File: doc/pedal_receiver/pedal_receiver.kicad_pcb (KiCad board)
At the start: 2 copper layers, 77 x 17.5 mm, 8 parts

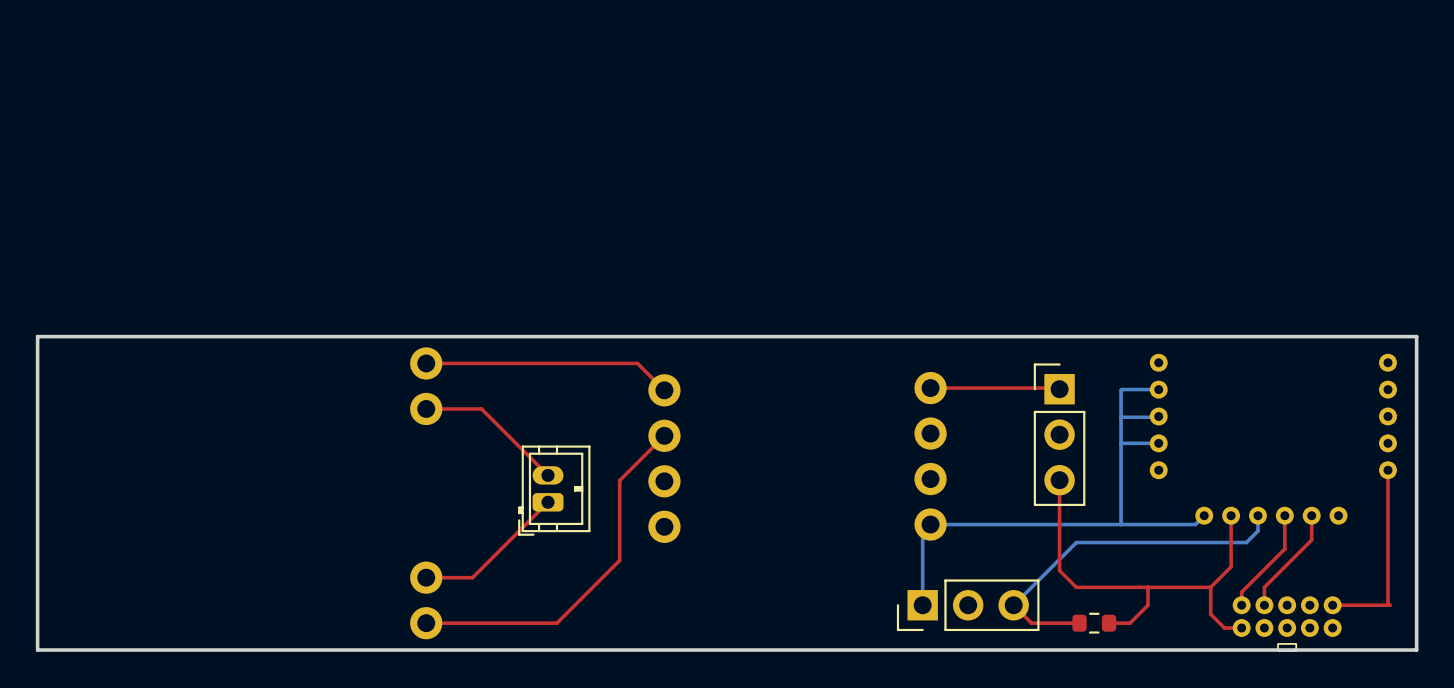
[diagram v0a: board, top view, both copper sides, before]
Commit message: g bluez
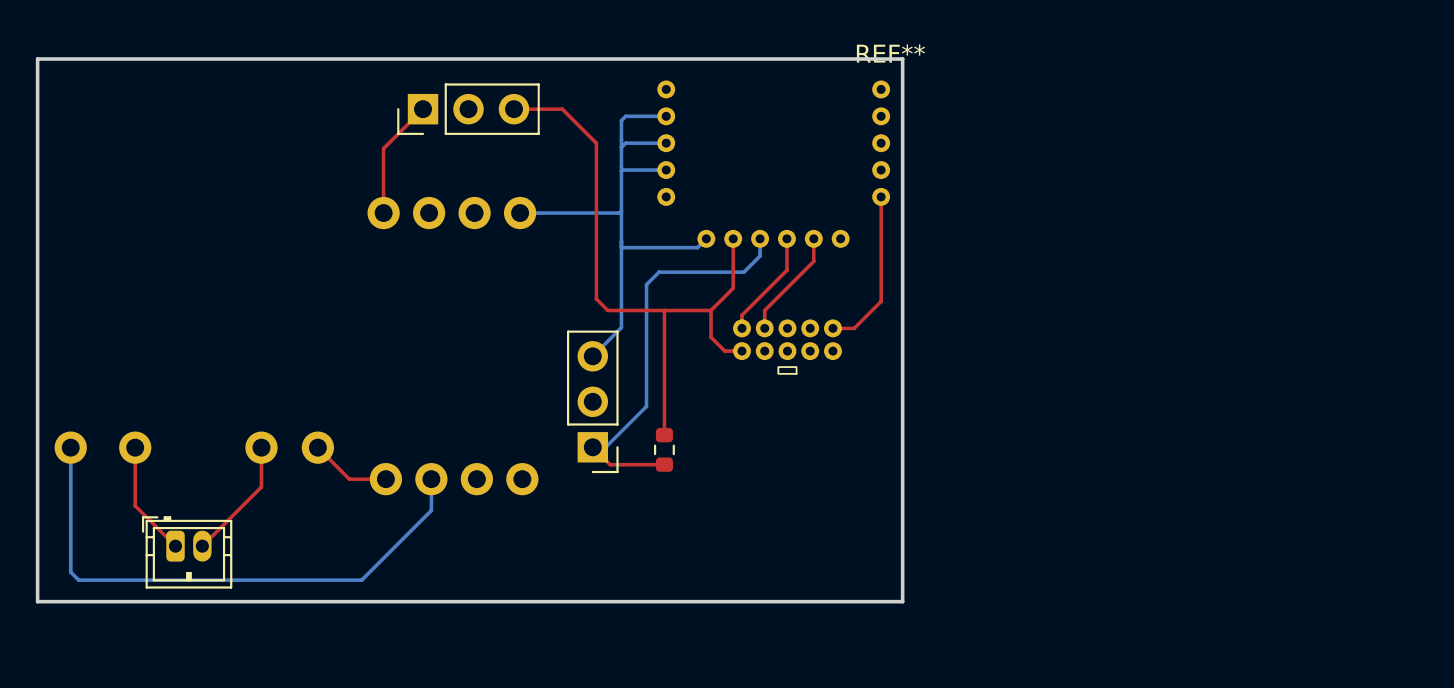
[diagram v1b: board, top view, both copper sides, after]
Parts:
- moved REF** 39.3 mm to (77.5, 32.3)
- moved REF** 31.9 mm to (97.1, 34.5)
- moved REF** 31.9 mm to (97.9, 45.8)
- moved REF** 26.3 mm to (87.0, 51.2), turned to 180 degrees
- moved REF** 25.9 mm to (91.0, 51.3), turned to -90 degrees
- moved REF** 20.9 mm to (63.7, 56.7), turned to 0 degrees
- moved J? 20.1 mm to (79.3, 45.6), turned to 90 degrees
- moved J? 12.4 mm to (64.4, 42.0), turned to -90 degrees
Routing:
- net (no net): track 162.6 -> 167.9 mm
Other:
- board size 77 x 17.5 mm -> 48.3 x 30.3 mm
